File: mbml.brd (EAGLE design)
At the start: 69.8 x 69.8 mm, 36 parts, among them K1 G5SB, Q1 2N2222, U1 REG_5V_SWITCHING_SI-8050E, X1 43160-1102, X10 CON_DB9VERT, X2 CON-2

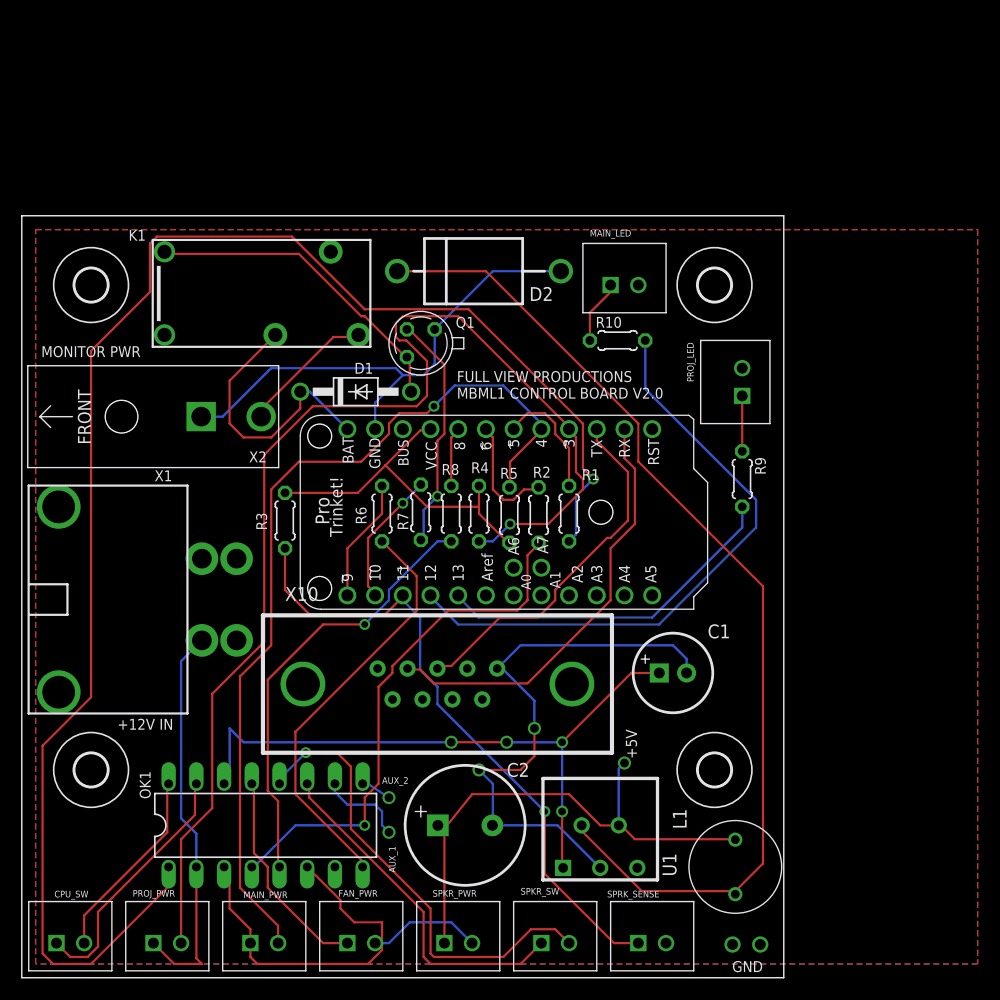
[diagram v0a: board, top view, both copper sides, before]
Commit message: Version 2.1, DRC OK
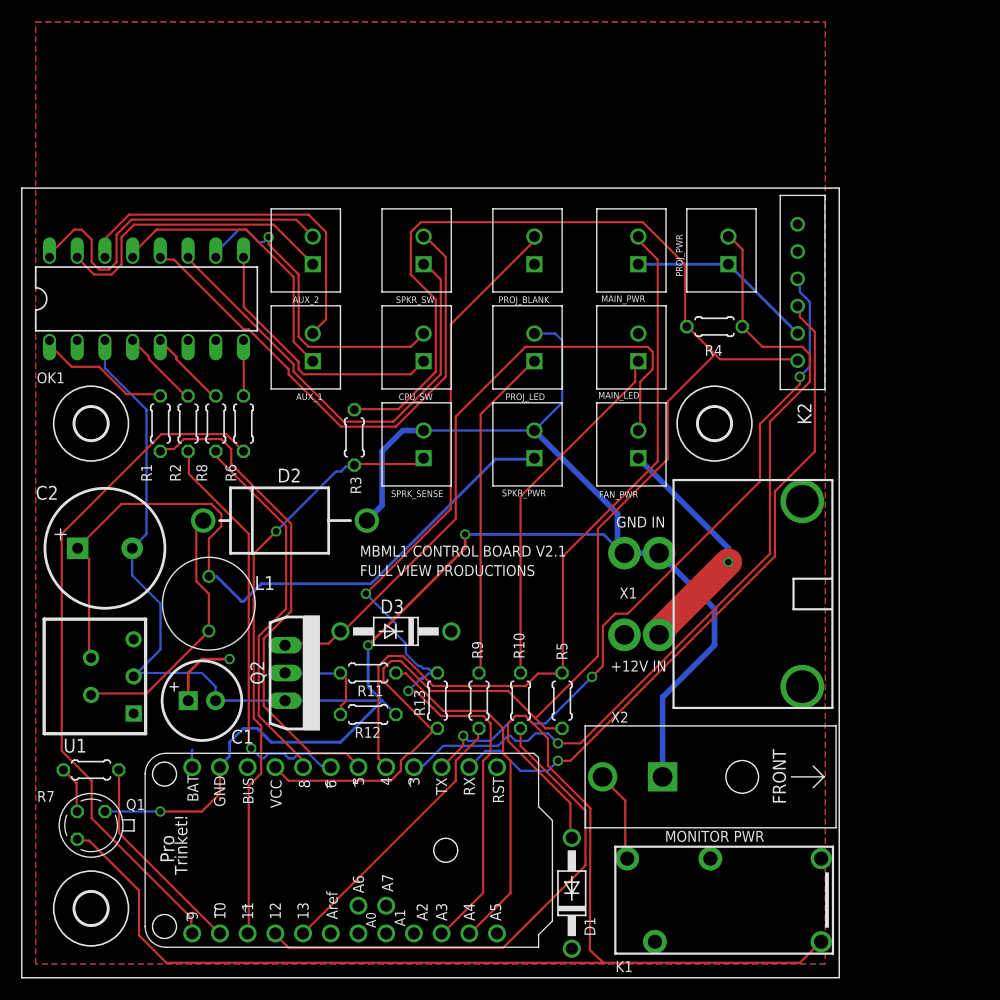
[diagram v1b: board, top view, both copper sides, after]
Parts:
- removed H3: MOUNT-HOLE3.0, holes:3,0
- removed X10: CON_DB9VERT, TinkerTech:D09P24A4GV00LF
- added AUX_1, AUX_2, PROJ_BLANK: CON-2B2B-XH-A(LF)(SN), FVP:CON_2-2.5MM_TH
- added D3: 1N4004, diode:DO41-10
- added K2: 68800611622, Wurth_Wire_to_Board_Connectors_rev15d:68800611622
- added Q2: IRLZ24LPBF, transistor-power:TO262-V
- added R11: 100, resistor:0204/5
- added R12, R13: 10k, resistor:0204/5
- R9: value 470 -> 1.8k
- moved PROJ_PWR 81.7 mm to (64.8, 66.7), turned to 90 degrees
- moved H2 80.8 mm to (6.35, 6.35), turned to 180 degrees
- moved MAIN_PWR 72.2 mm to (56.5, 66.7), turned to 90 degrees
- moved K1 71.5 mm to (65.7, 7.11), turned to 0 degrees
- moved X2 65.8 mm to (66.0, 18.4), turned to 90 degrees
- moved H1 65.4 mm to (63.5, 50.8), turned to 180 degrees
- moved H4 65.4 mm to (6.35, 50.8), turned to 180 degrees
- moved SPKR_SW 64.6 mm to (36.8, 66.7), turned to 90 degrees
- moved CPU_SW 63.5 mm to (36.8, 57.8), turned to 90 degrees
- moved L1 54.0 mm to (17.1, 34.3)
- moved Q1 53.5 mm to (6.35, 14.0)
- moved FAN_PWR 52.3 mm to (56.5, 48.9), turned to 90 degrees
- moved SPRK_SENSE 50.3 mm to (36.8, 48.9), turned to 90 degrees
- moved D1 50.1 mm to (50.4, 7.75), turned to 90 degrees
- moved OK1 49.5 mm to (11.4, 62.2)
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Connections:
- removed net AUX_1: OK1.10
- removed net AUX_2: OK1.9
- new net N$10: Q2.2, R11.1, R12.1
- new net N$12: AUX_1.P$2, OK1.14
- new net N$13: AUX_1.P$1, OK1.13
- new net N$18: CPU_SW.P$1, OK1.9
- new net N$9: D3.A, FAN_PWR.P$2, Q2.1
- net +12V: now also D3.C, FAN_PWR.P$1; no longer OK1.14
- net A3: now also PROJ_BLANK.P$2, R13.1
- net A4: now also R11.2
- net GND: now also K2.5, PROJ_BLANK.P$1, Q2.3, R12.2; no longer FAN_PWR.P$2, X10.5
- net MCU_VCC: now also K2.6, R13.2
- net N$14: now also CPU_SW.P$2, OK1.10; no longer FAN_PWR.P$1, OK1.13
- net N$15: now also AUX_2.P$1; no longer CPU_SW.P$1
- net N$16: now also AUX_2.P$2; no longer CPU_SW.P$2
- net RX: now also K2.4; no longer X10.2
- net TX: now also K2.3; no longer X10.3
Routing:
- net N$8: track 145.1 -> 12.5 mm, vias 1 -> 0
- net MCU_VCC: track 32.4 -> 152.4 mm
- net TRANS_COLLECTOR: track 29.7 -> 116.5 mm
- net A3: track 0.00 -> 83.1 mm, vias 0 -> 2
- net N$1: track 93.8 -> 24.2 mm
- net N$9: track 0.00 -> 58.8 mm
- net +12V: track 84.6 -> 30.7 mm, vias 4 -> 2
- net D9: track 11.3 -> 62.7 mm
- net GND: track 180.4 -> 222.3 mm, vias 4 -> 3
- net N$7: track 48.1 -> 7.37 mm, vias 1 -> 0
- net D5: track 11.2 -> 45.3 mm
- net D3: track 111.4 -> 77.8 mm
- net N$12: track 0.00 -> 33.4 mm
- net N$17: track 38.4 -> 5.08 mm
- net N$2: track 40.3 -> 7.37 mm, vias 1 -> 0
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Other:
- board size 69.8 x 69.8 mm -> 74.9 x 72.4 mm
- board text added: "GND IN"
- board text added: "MBML1 CONTROL BOARD V2.1"
- board text removed: "+5V"
- board text removed: "AUX_1"
- board text removed: "AUX_2"
- board text removed: "GND"
- board text removed: "MBML1 CONTROL BOARD V2.0"
